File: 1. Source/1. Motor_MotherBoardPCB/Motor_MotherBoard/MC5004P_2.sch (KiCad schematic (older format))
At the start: 3 parts, among them U2 MC5004P, U4 CON_6pin_motor

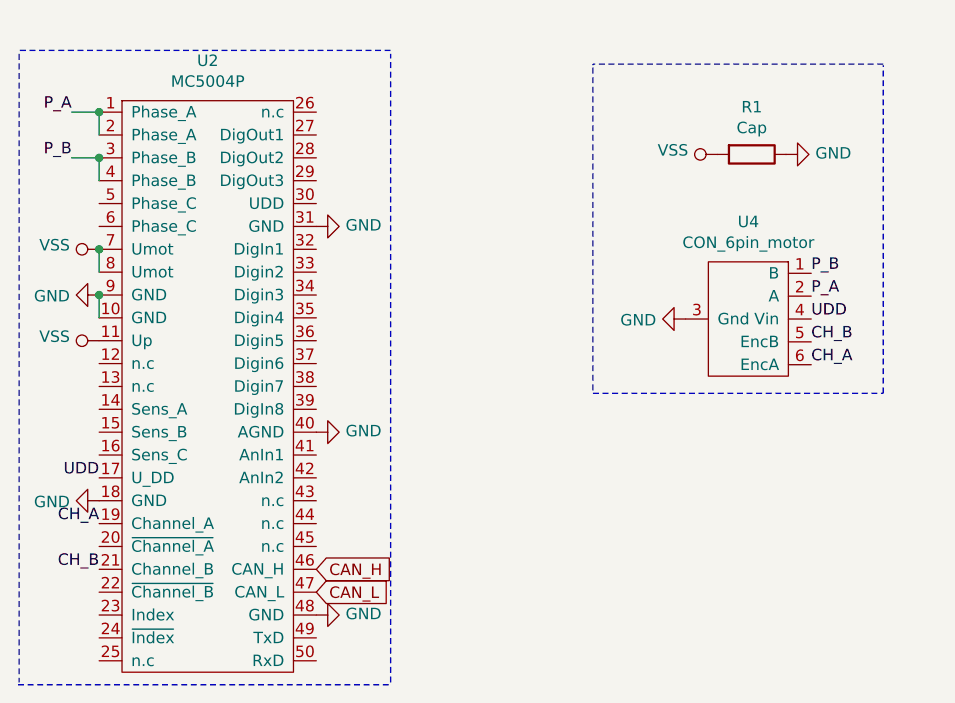
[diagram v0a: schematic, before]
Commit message: PCB_MotorMotherBoard
PCB_MotorMotherBoard
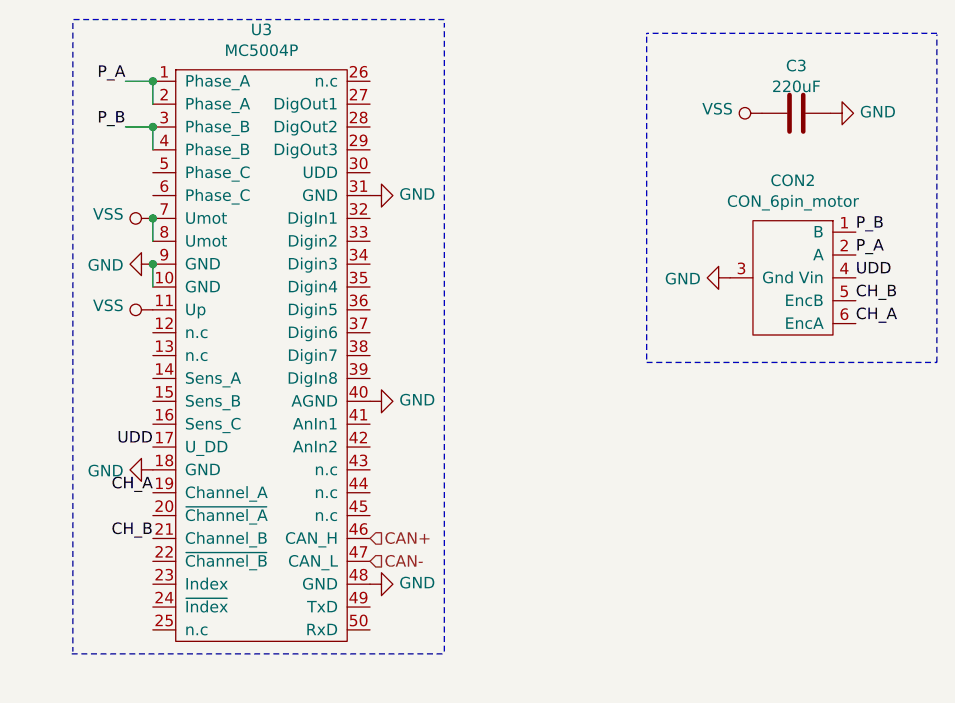
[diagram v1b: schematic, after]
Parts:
- removed R1: Cap, Resistor_THT:R_Axial_DIN0414_L11.9mm_D4.5mm_P5.08mm_Vertical, symbol Device:R
- removed U2: MC5004P, BC_Motor_Driver:MC5004P, symbol BC_Motor_Drivers:MC5004P
- removed U4: CON_6pin_motor, Connector_IDC:IDC-Header_2x03_P2.54mm_Vertical, symbol BC_Connectors:CON_6pin_motor
- added C3: 220uF, Capacitor_THT:CP_Radial_D8.0mm_P3.80mm, symbol Device:C
- added CON2: CON_6pin_motor, Connector_IDC:IDC-Header_2x03_P2.54mm_Vertical, symbol BC_Connectors:CON_6pin_motor
- added U3: MC5004P, BC_Motor_Driver:MC5004P, symbol BC_Motor_Drivers:MC5004P
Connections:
- net CH_A: now also CON2.6 (EncA), U3.19 (Channel_A)
- net CH_B: now also CON2.5 (EncB), U3.21 (Channel_B)
- net GND: now also C3.1, CON2.3 (Gnd), U3.10 (GND), U3.18 (GND), U3.31 (GND), U3.40 (AGND), U3.48 (GND), U3.9 (GND)
- net P_A: now also CON2.2 (A), U3.1 (Phase_A), U3.2 (Phase_A)
- net P_B: now also CON2.1 (B), U3.3 (Phase_B), U3.4 (Phase_B)
- net UDD: now also CON2.4 (Vin), U3.17 (U_DD)
- net VSS: now also C3.2, U3.11 (Up), U3.7 (Umot), U3.8 (Umot)
- new net CAN+: U3.46 (CAN_H)
- new net CAN-: U3.47 (CAN_L)
